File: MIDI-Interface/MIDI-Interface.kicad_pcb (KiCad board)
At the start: 2 copper layers, 160.1 x 128.2 mm, 80 parts, among them J1 Conn_01x06_Pin, J2 Conn_01x01_Pin, J3 Conn_01x01_Pin, J4 Conn_01x14_Pin, J5 Conn_01x14_Pin, SW1 RotaryEncoder_Switch, U1 TL074, U10 Aux_flush, U11 Aux_flush, U12 Aux_flush, U13 Aux_flush, U2 L7806, U3 EL817, U4 TL072, U5 TL074, U6 Aux_flush, U7 Aux_flush, U8 Aux_flush, U9 Aux_flush

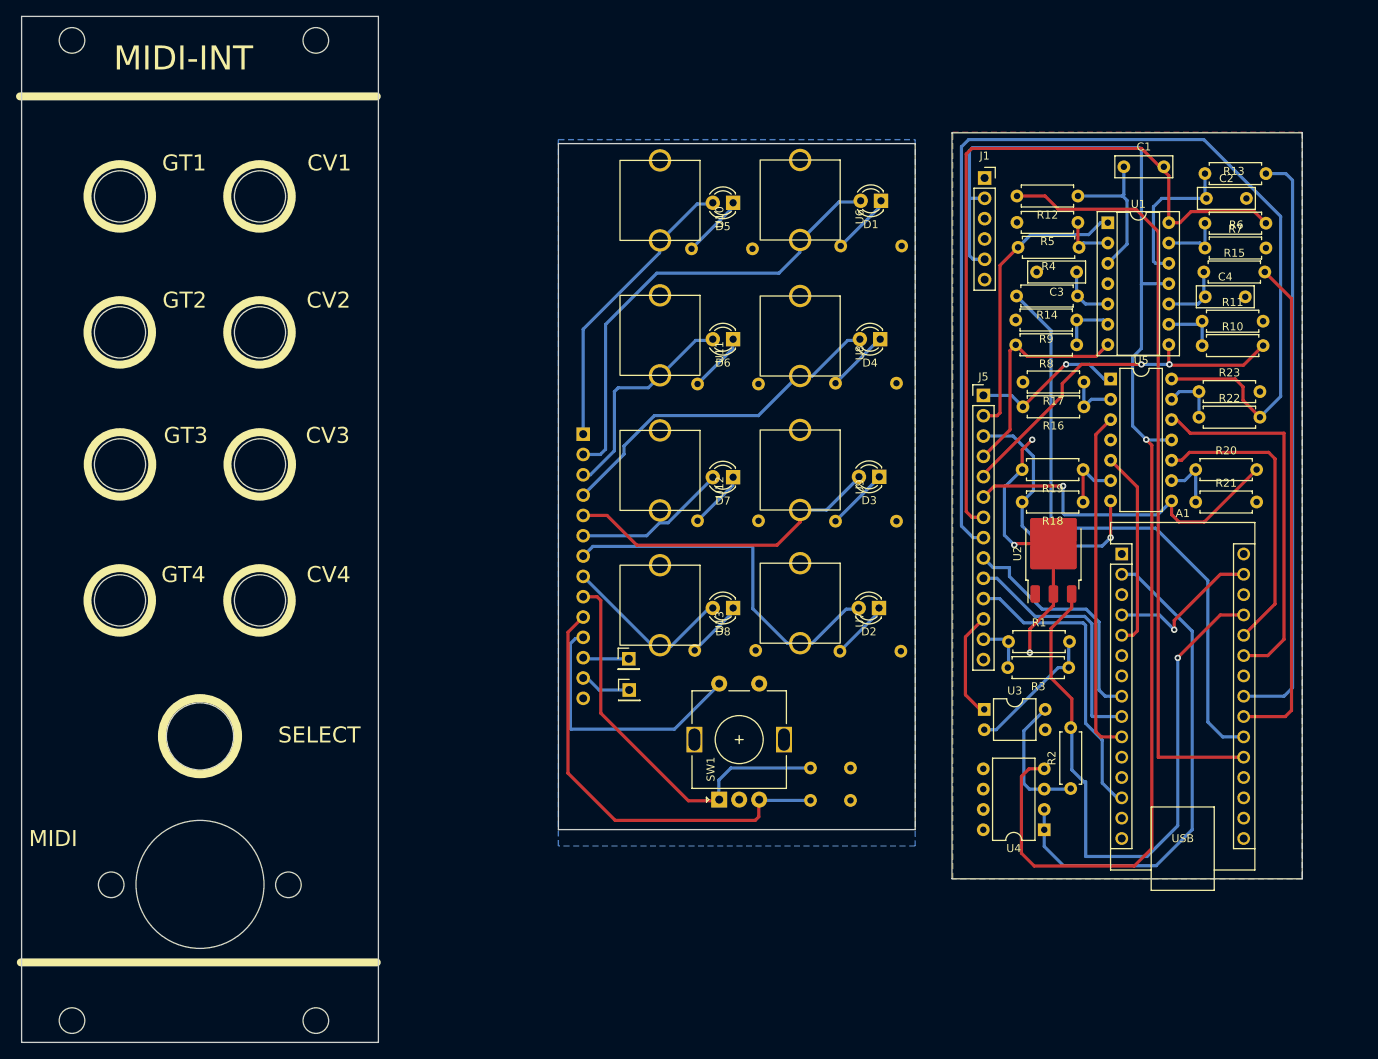
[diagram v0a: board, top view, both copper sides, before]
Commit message: Add files via upload
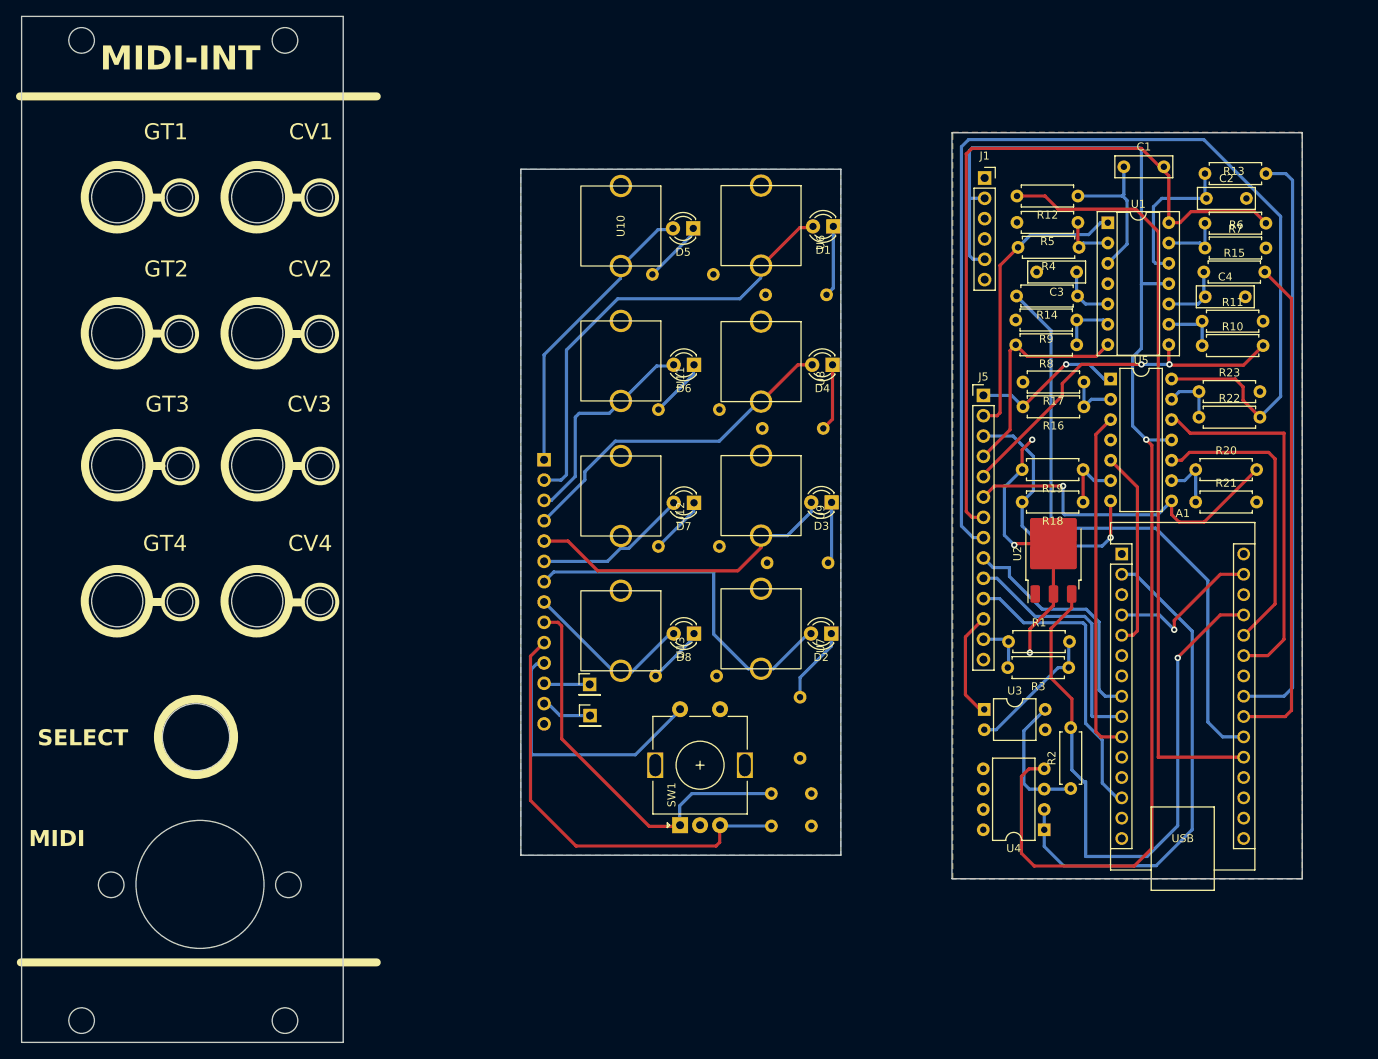
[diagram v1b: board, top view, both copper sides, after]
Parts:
- added REF**: MountingHole_3.2mm_M3, MountingHole:MountingHole_3.2mm_M3, F.Cu at (72.5, 103.2)
- added REF**: MountingHole_3.2mm_M3, MountingHole:MountingHole_3.2mm_M3, F.Cu at (72.5, 52.6)
- added REF**: MountingHole_3.2mm_M3, MountingHole:MountingHole_3.2mm_M3, F.Cu at (90.0, 69.7)
- added REF**: MountingHole_3.2mm_M3, MountingHole:MountingHole_3.2mm_M3, F.Cu at (90.0, 52.6)
- added REF**: MountingHole_3.2mm_M3, MountingHole:MountingHole_3.2mm_M3, F.Cu at (90.0, 103.2)
- added REF**: MountingHole_3.2mm_M3, MountingHole:MountingHole_3.2mm_M3, F.Cu at (90.0, 86.2)
- added REF**: MountingHole_3.2mm_M3, MountingHole:MountingHole_3.2mm_M3, F.Cu at (72.5, 86.2)
- added REF**: MountingHole_3.2mm_M3, MountingHole:MountingHole_3.2mm_M3, F.Cu at (72.5, 69.7)
- moved R25 7.61 mm to (150.0, 115.1), turned to -90 degrees
- moved D1 6.76 mm to (154.2, 56.2)
- moved D2 6.76 mm to (153.9, 107.2)
- moved D3 6.76 mm to (153.9, 90.8)
- moved D4 6.76 mm to (154.1, 73.5)
- moved R24 6.35 mm to (153.3, 64.8), turned to 180 degrees
- moved D5 5.92 mm to (136.7, 56.5)
- moved R27 5.85 mm to (152.9, 81.5), turned to 180 degrees
- moved C5 5.84 mm to (146.4, 127.2)
- moved R31 5.84 mm to (131.9, 112.5)
- moved U7 5.84 mm to (145.1, 106.5)
- moved U8 5.84 mm to (145.1, 73.2)
- moved U9 5.84 mm to (145.1, 89.9)
- moved U6 5.84 mm to (145.1, 56.1)
- moved C6 5.84 mm to (146.4, 131.2)
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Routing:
- net Net-(D2-K): track 7.25 -> 9.57 mm
- net CV4: track 139.6 -> 138.1 mm
- net Net-(D1-K): track 7.56 -> 8.90 mm
- net CV2: track 71.5 -> 70.3 mm
- net CV1: track 94.0 -> 93.0 mm
- net Net-(D4-K): track 7.75 -> 8.43 mm
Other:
- outline, holes or cut-outs redrawn

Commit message: Add files via upload
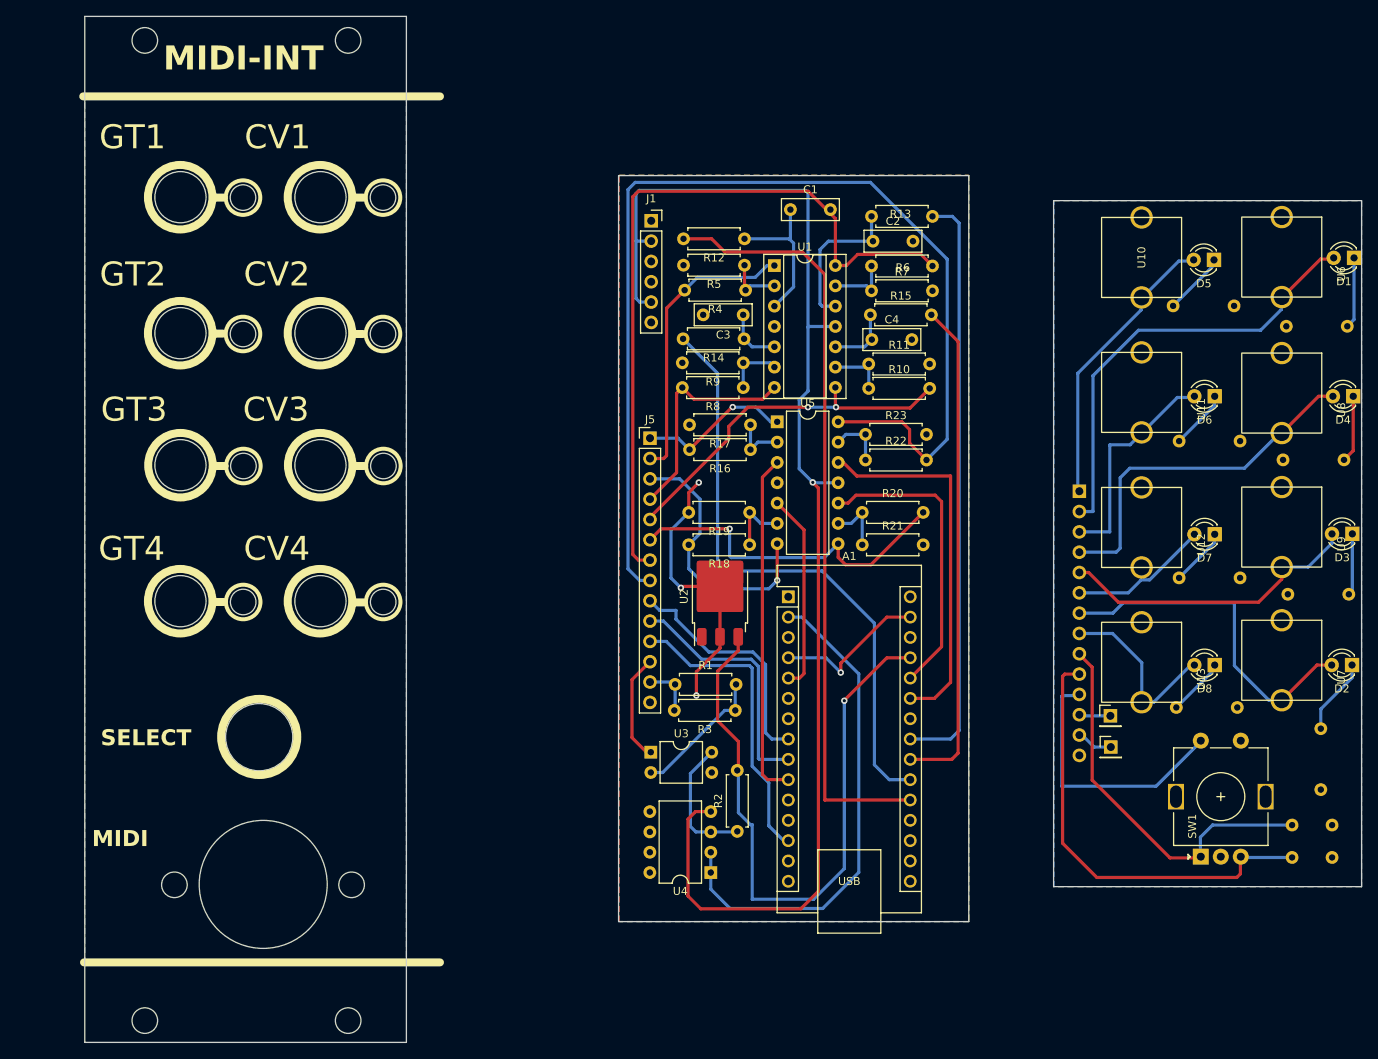
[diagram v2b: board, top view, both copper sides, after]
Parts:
- removed the REF** at (72.5, 103.2)
- removed the REF** at (82.2, 69.6)
- removed the REF** at (64.7, 69.6)
- removed the REF** at (86.0, 138.6)
- removed the REF** at (72.5, 52.6)
- removed the REF** at (85.6, 155.5)
- removed the REF** at (82.2, 52.6)
- removed the REF** at (90.0, 69.7)
- removed the REF** at (60.2, 155.5)
- removed the REF** at (90.0, 52.6)
- removed the REF** at (64.7, 103.1)
- removed the REF** at (82.2, 103.1)
- removed the REF** at (90.0, 103.2)
- removed the REF** at (85.6, 33.0)
- removed the REF** at (64.7, 52.6)
- removed the REF** at (60.2, 33.0)
- removed the REF** at (90.0, 86.2)
- removed the REF** at (72.5, 86.2)
- removed the REF** at (63.9, 138.6)
- removed the REF** at (64.7, 86.1)
- removed the REF** at (72.5, 69.7)
- removed the REF** at (82.2, 86.1)
- added REF**: MountingHole_3.2mm_M3, MountingHole:MountingHole_3.2mm_M3, F.Cu at (93.5, 33.0)
- added REF**: MountingHole_6.4mm_M6, MountingHole:MountingHole_6.4mm_M6, F.Cu at (90.1, 52.6)
- added REF**: MountingHole_3.2mm_M3, MountingHole:MountingHole_3.2mm_M3, F.Cu at (80.4, 103.2)
- added REF**: MountingHole_3.2mm_M3, MountingHole:MountingHole_3.2mm_M3, F.Cu at (93.5, 155.5)
- added REF**: MountingHole_3.2mm_M3, MountingHole:MountingHole_3.2mm_M3, F.Cu at (80.4, 69.7)
- added REF**: MountingHole_3.2mm_M3, MountingHole:MountingHole_3.2mm_M3, F.Cu at (68.1, 155.5)
- added REF**: MountingHole_3.2mm_M3, MountingHole:MountingHole_3.2mm_M3, F.Cu at (94.0, 138.6)
- added REF**: MountingHole_6.4mm_M6, MountingHole:MountingHole_6.4mm_M6, F.Cu at (72.6, 86.1)
- added REF**: MountingHole_3.2mm_M3, MountingHole:MountingHole_3.2mm_M3, F.Cu at (68.1, 33.0)
- added REF**: MountingHole_6.4mm_M6, MountingHole:MountingHole_6.4mm_M6, F.Cu at (72.6, 52.6)
- added REF**: MountingHole_6.4mm_M6, MountingHole:MountingHole_6.4mm_M6, F.Cu at (72.6, 69.6)
- added REF**: MountingHole_3.2mm_M3, MountingHole:MountingHole_3.2mm_M3, F.Cu at (71.8, 138.6)
- added REF**: MountingHole_3.2mm_M3, MountingHole:MountingHole_3.2mm_M3, F.Cu at (97.9, 69.7)
- added REF**: MountingHole_3.2mm_M3, MountingHole:MountingHole_3.2mm_M3, F.Cu at (97.9, 86.2)
- added REF**: MountingHole_3.2mm_M3, MountingHole:MountingHole_3.2mm_M3, F.Cu at (80.4, 52.6)
- added REF**: MountingHole_6.4mm_M6, MountingHole:MountingHole_6.4mm_M6, F.Cu at (90.1, 69.6)
- added REF**: MountingHole_3.2mm_M3, MountingHole:MountingHole_3.2mm_M3, F.Cu at (97.9, 52.6)
- added REF**: MountingHole_6.4mm_M6, MountingHole:MountingHole_6.4mm_M6, F.Cu at (72.6, 103.1)
- added REF**: MountingHole_3.2mm_M3, MountingHole:MountingHole_3.2mm_M3, F.Cu at (97.9, 103.2)
- added REF**: MountingHole_6.4mm_M6, MountingHole:MountingHole_6.4mm_M6, F.Cu at (90.1, 86.1)
- added REF**: MountingHole_6.4mm_M6, MountingHole:MountingHole_6.4mm_M6, F.Cu at (90.1, 103.1)
- added REF**: MountingHole_3.2mm_M3, MountingHole:MountingHole_3.2mm_M3, F.Cu at (80.4, 86.2)
- moved J4 67.0 mm to (184.9, 89.4)
- moved J2 65.2 mm to (188.8, 117.4)
- moved C5 65.2 mm to (211.5, 131.1)
- moved C6 65.2 mm to (211.5, 135.1)
- moved D1 65.2 mm to (219.3, 60.2)
- moved D2 65.2 mm to (219.0, 111.1)
- moved D3 65.2 mm to (219.0, 94.7)
- moved D4 65.2 mm to (219.2, 77.5)
- moved D5 65.2 mm to (201.8, 60.4)
- moved D6 65.2 mm to (201.8, 77.5)
- moved D7 65.2 mm to (201.8, 94.7)
- moved D8 65.2 mm to (201.8, 111.1)
- moved R24 65.2 mm to (218.4, 68.7)
- moved R25 65.2 mm to (215.1, 119.0)
- moved R26 65.2 mm to (218.6, 102.2)
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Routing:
- net CV2: track 70.3 -> 73.0 mm
- net GT3: track 62.8 -> 61.0 mm
- net CV3: track 85.4 -> 83.6 mm
- net ENCA: track 80.5 -> 78.7 mm
- net CV4: track 138.1 -> 136.9 mm
- net MIDI-4: track 18.6 -> 17.5 mm
- net MIDI-5: track 12.2 -> 11.1 mm
- net CV1: track 93.0 -> 92.0 mm
- net GT4: track 156.9 -> 157.9 mm
- net SW: track 71.9 -> 71.1 mm
- net ENCB: track 86.3 -> 86.9 mm
- net GT1: track 56.0 -> 55.4 mm
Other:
- board size 160.1 x 128.2 mm -> 159.6 x 128.2 mm
